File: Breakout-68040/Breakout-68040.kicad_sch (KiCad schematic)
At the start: 46 parts, among them IC1 DS1232S+, IC2 ATF22V10C-7PU, J1 Conn_02x32_Odd_Even, J10 Conn_01x03_Pin, J2 Conn_01x02_Pin, J3 Conn_01x32_Pin, J4 Conn_02x32_Odd_Even, J5 Conn_02x16_Odd_Even, J6 Conn_01x16_Pin, J7 Conn_01x08_Pin, J8 Conn_02x12_Odd_Even, J9 Conn_01x03_Pin, SW1 Reset, U1 MC680LC40, X1 SG-615

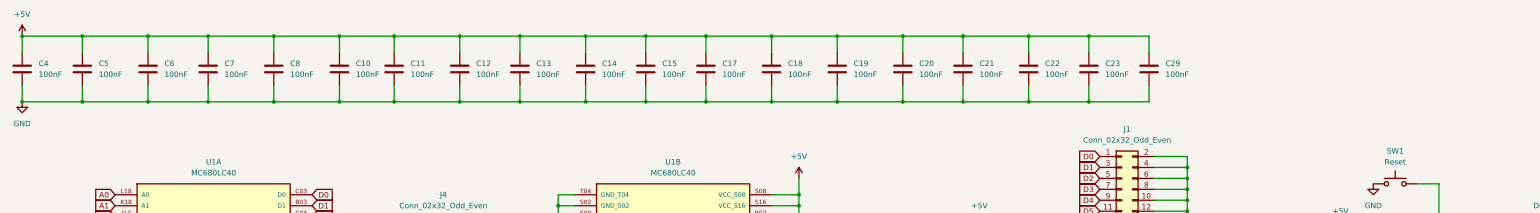
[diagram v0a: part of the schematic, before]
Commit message: Sent to jclpcb
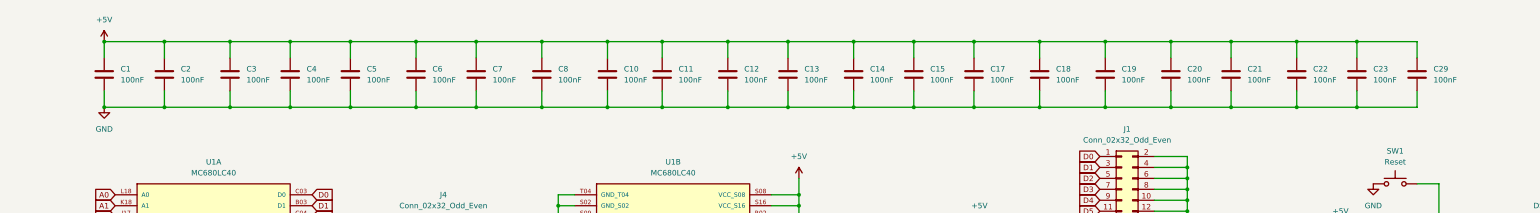
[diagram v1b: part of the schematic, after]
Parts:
- added C1, C2, C3: 100nF, Capacitor_SMD:C_0805_2012Metric_Pad1.18x1.45mm_HandSolder, symbol Device:C
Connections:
- net +5V: now also C1.1, C2.1, C3.1
- net GND: now also C1.2, C2.2, C3.2
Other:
- moved on the sheet: C10, C11, C12, C13, C14, C15, C17, C18, C19, C20, C21, C22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

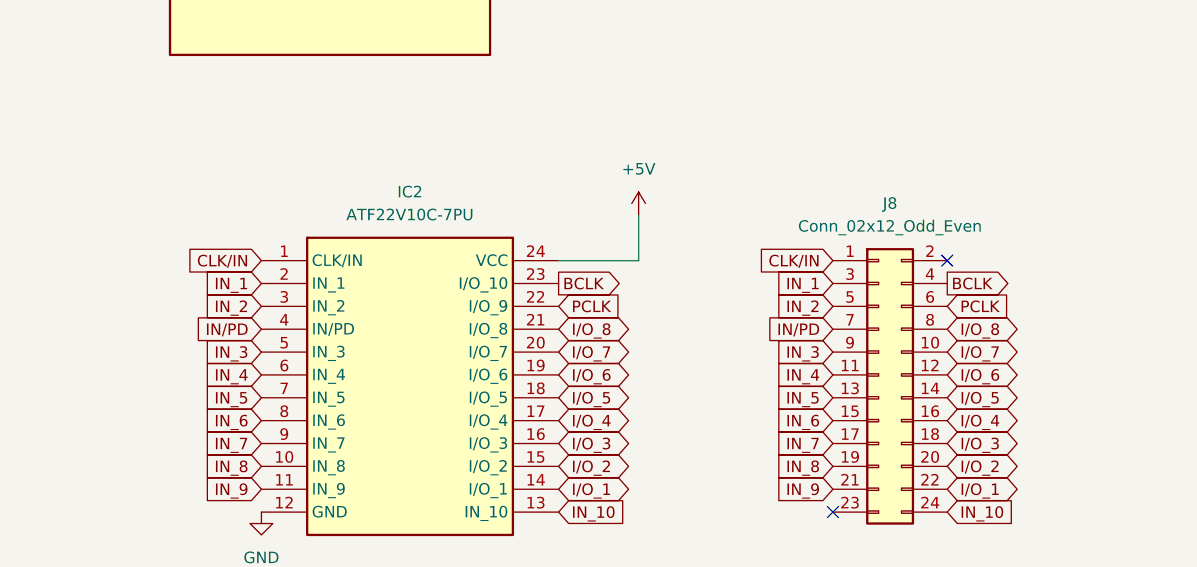
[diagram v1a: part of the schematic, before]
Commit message: Mothballing
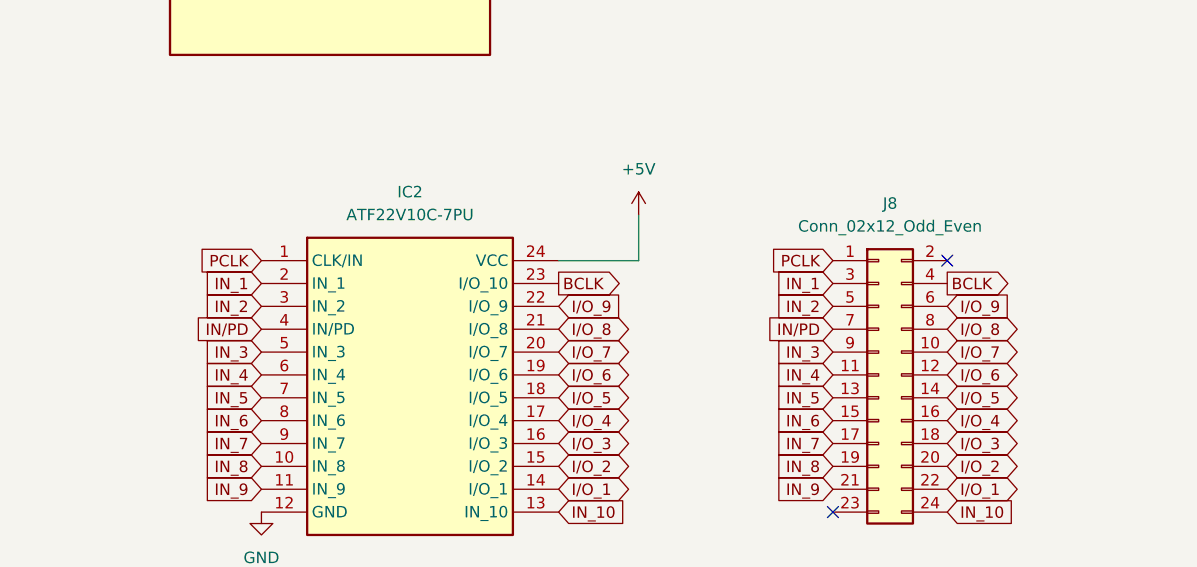
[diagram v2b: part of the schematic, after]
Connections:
- net CLK/IN is gone; now on net PCLK: IC2.1 (CLK/IN), J8.1 (Pin_1)
- net PCLK: no longer IC2.22 (I/O_9), J8.6 (Pin_6)
- new net I/O_9: IC2.22 (I/O_9), J8.6 (Pin_6)
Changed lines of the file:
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@@
 		)
 	)
-	(global_label "PCLK"
+	(global_label "I{slash}O_9"
 		(shape input)
 		(at 195.58 251.46 0)
@@
 		)
 		(property "Intersheetrefs" "${INTERSHEET_REFS}"
-			(at 203.4033 251.46 0)
+			(at 204.0081 251.46 0)
 			(effects
 				(font
@@
 		)
 	)
-	(global_label "PCLK"
+	(global_label "I{slash}O_9"
 		(shape input)
 		(at 238.76 251.46 0)
@@
 		)
 		(property "Intersheetrefs" "${INTERSHEET_REFS}"
-			(at 246.5833 251.46 0)
+			(at 247.1881 251.46 0)
 			(effects
 				(font
@@
 		)
 	)
-	(global_label "CLK{slash}IN"
+	(global_label "PCLK"
 		(shape input)
 		(at 162.56 246.38 180)
@@
 		)
 		(property "Intersheetrefs" "${INTERSHEET_REFS}"
-			(at 152.7409 246.38 0)
+			(at 154.7367 246.38 0)
 			(effects
 				(font
@@
 		)
 	)
-	(global_label "CLK{slash}IN"
+	(global_label "PCLK"
 		(shape input)
 		(at 226.06 246.38 180)
@@
 		)
 		(property "Intersheetrefs" "${INTERSHEET_REFS}"
-			(at 216.2409 246.38 0)
-			(effects
-				(font
+			(at 218.2367 246.38 0)
+			(effects
+				(font
